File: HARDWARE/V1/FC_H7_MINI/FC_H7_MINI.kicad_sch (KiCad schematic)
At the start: 26 parts, among them Q1 2N7002KQBZ, U2 STM32G473CEUx, Y2 CSTNE8M00GH5C000R0

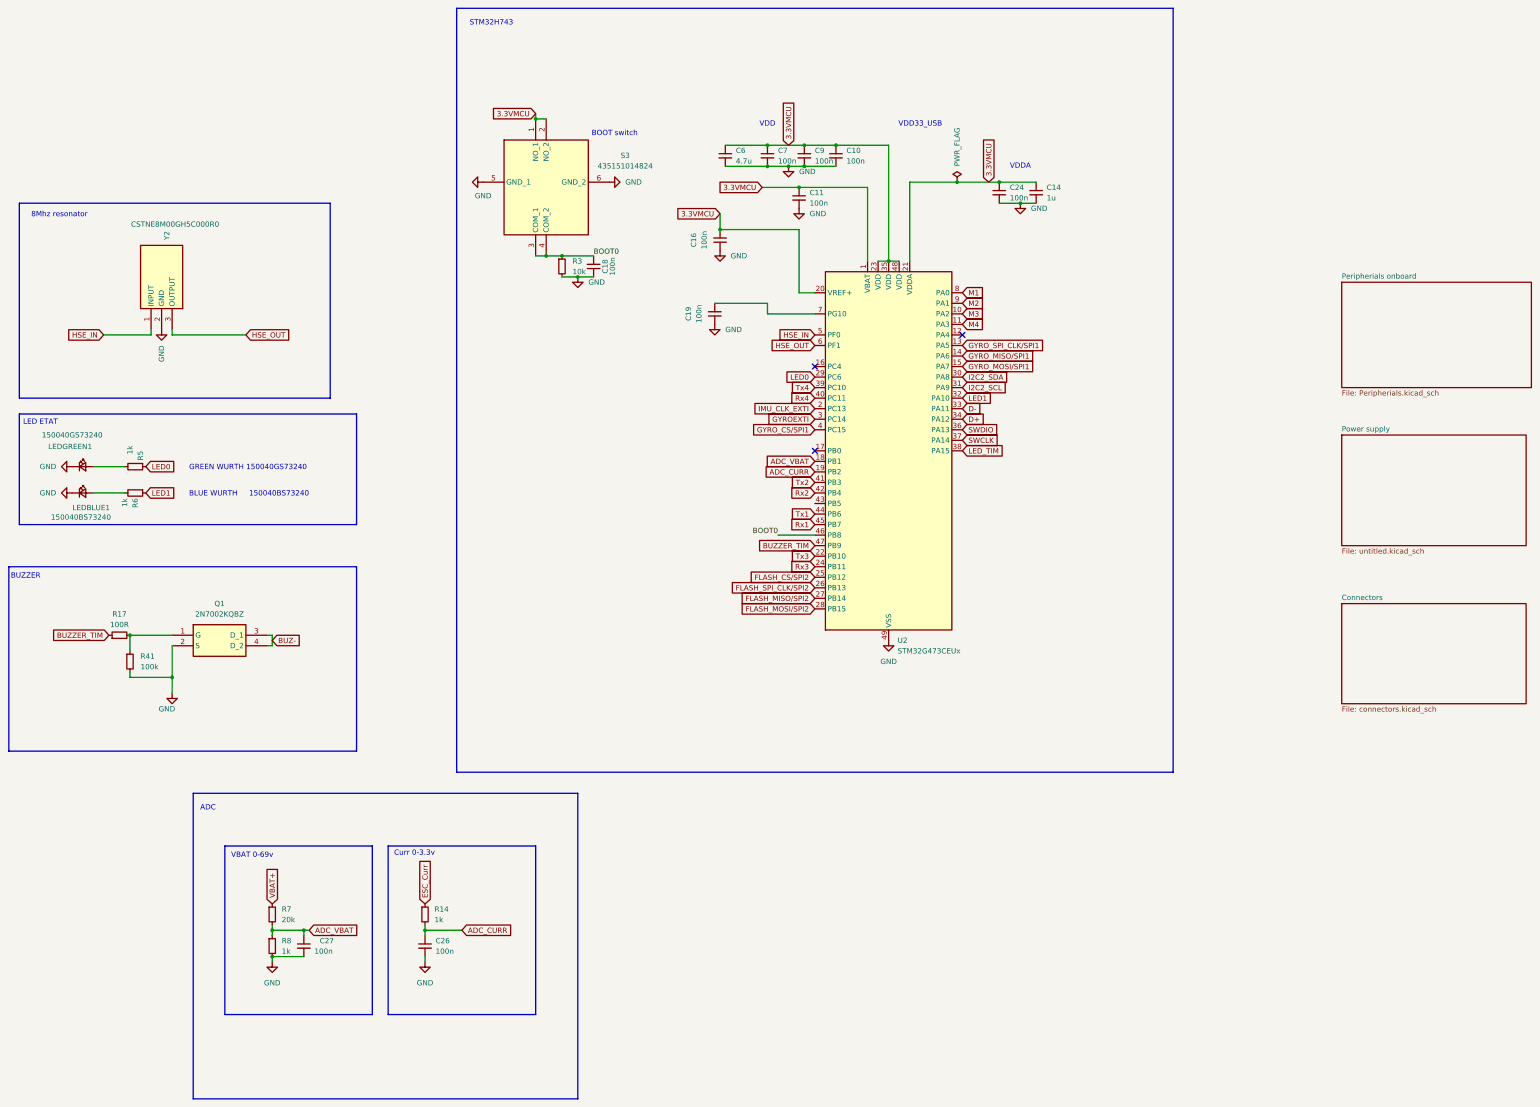
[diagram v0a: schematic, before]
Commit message: up
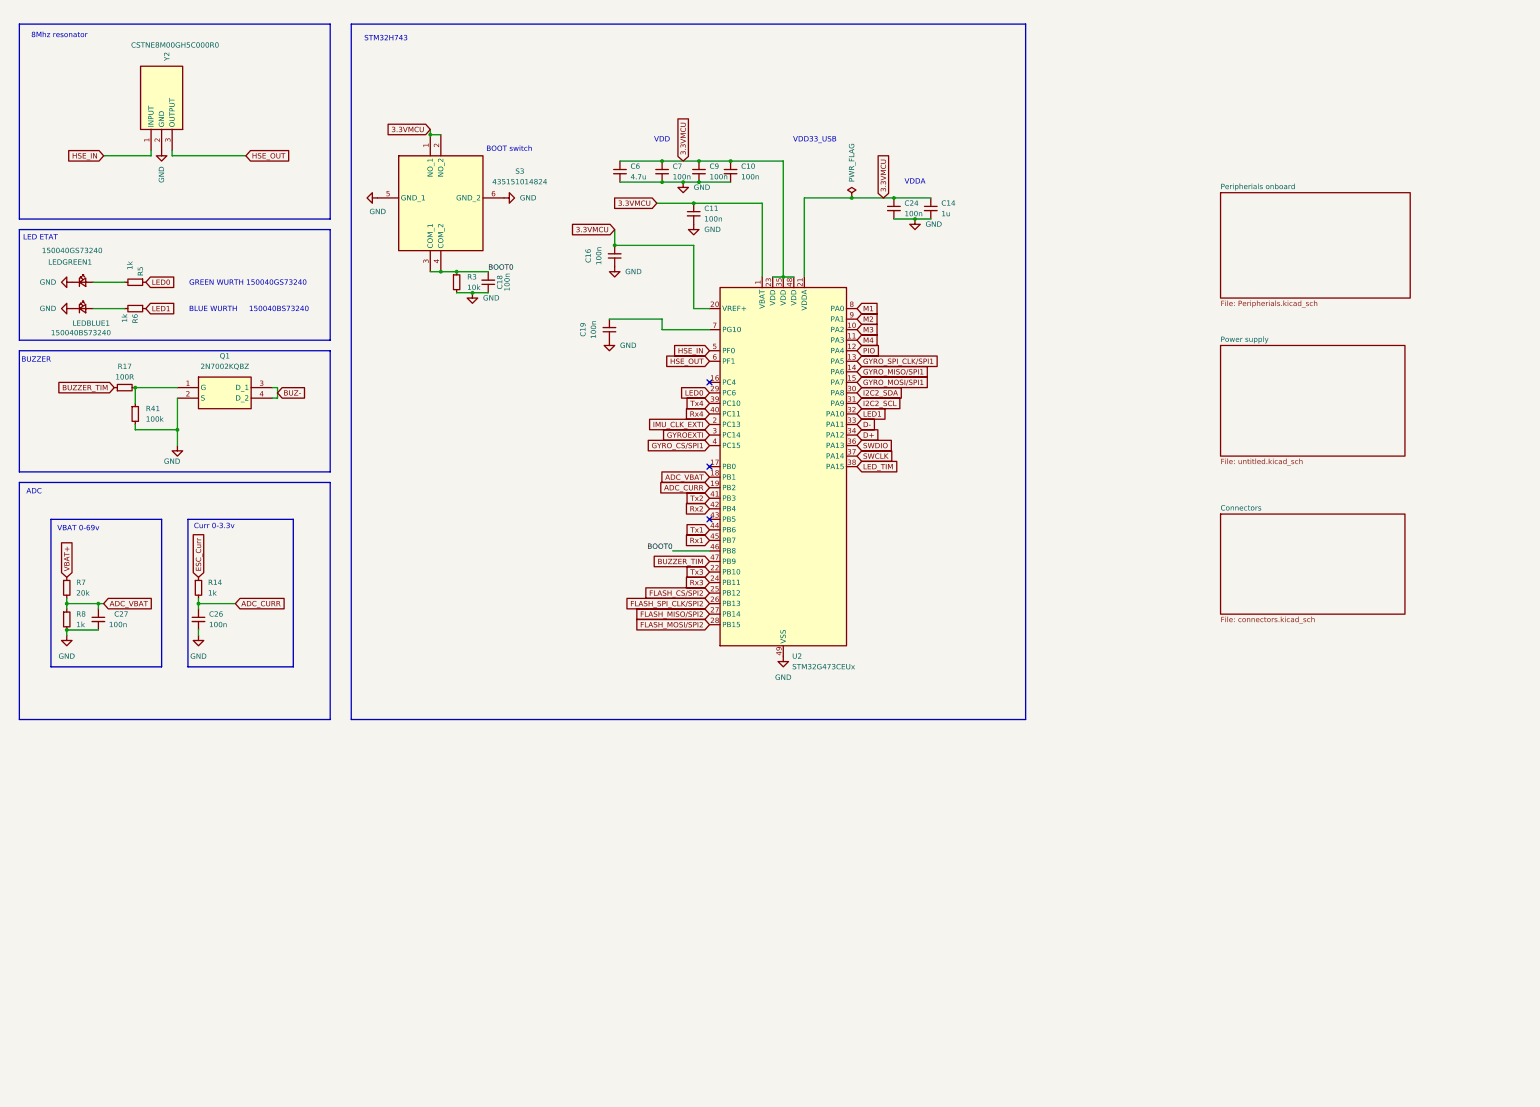
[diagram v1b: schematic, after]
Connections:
- net PIO: now reaches U2.12 (PA4)
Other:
- moved on the sheet: C10, C11, C14, C16, C18, C19, C24, C26, C27, C6, C7, C9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
